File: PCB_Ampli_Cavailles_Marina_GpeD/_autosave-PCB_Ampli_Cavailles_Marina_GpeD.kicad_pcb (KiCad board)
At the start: 2 copper layers, 52 parts, among them J2 Conn_01x02, J3 Conn_01x03, Q1 2N2907, Q10 TIP32, Q11 BD138, Q12 TIP31, Q13 2N2222, Q2 2N2907, Q3 2N2907, Q4 2N2222, Q5 2N2222, Q6 2N2907, Q7 2N2907, Q8 BD139, Q9 BD139, U1 Relay_1CT, U2 Jack_Mono

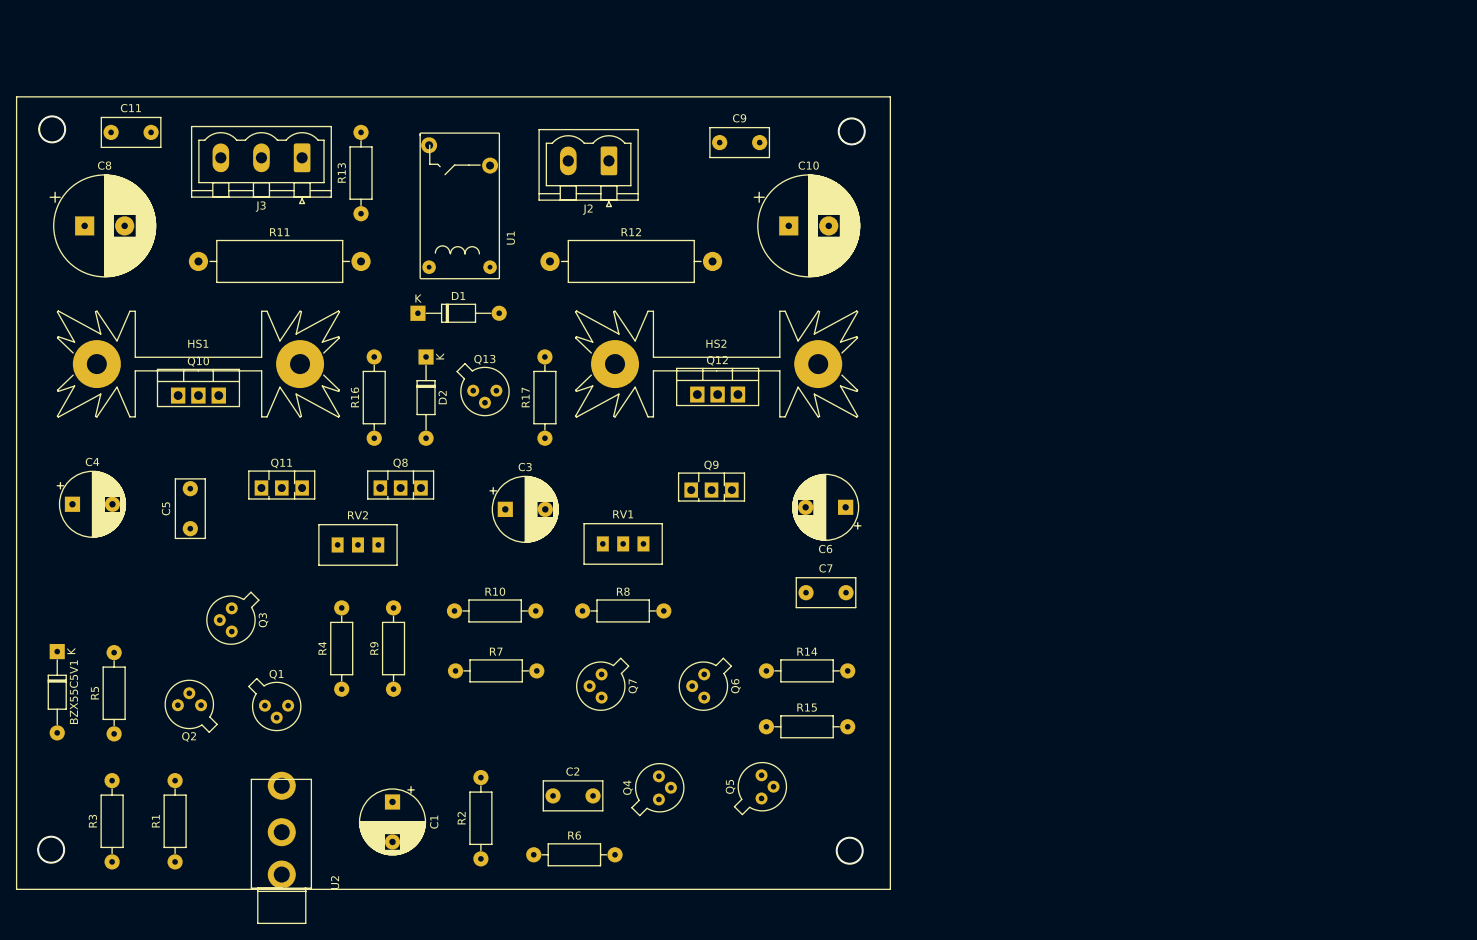
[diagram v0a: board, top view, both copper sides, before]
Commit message: PCB modifié
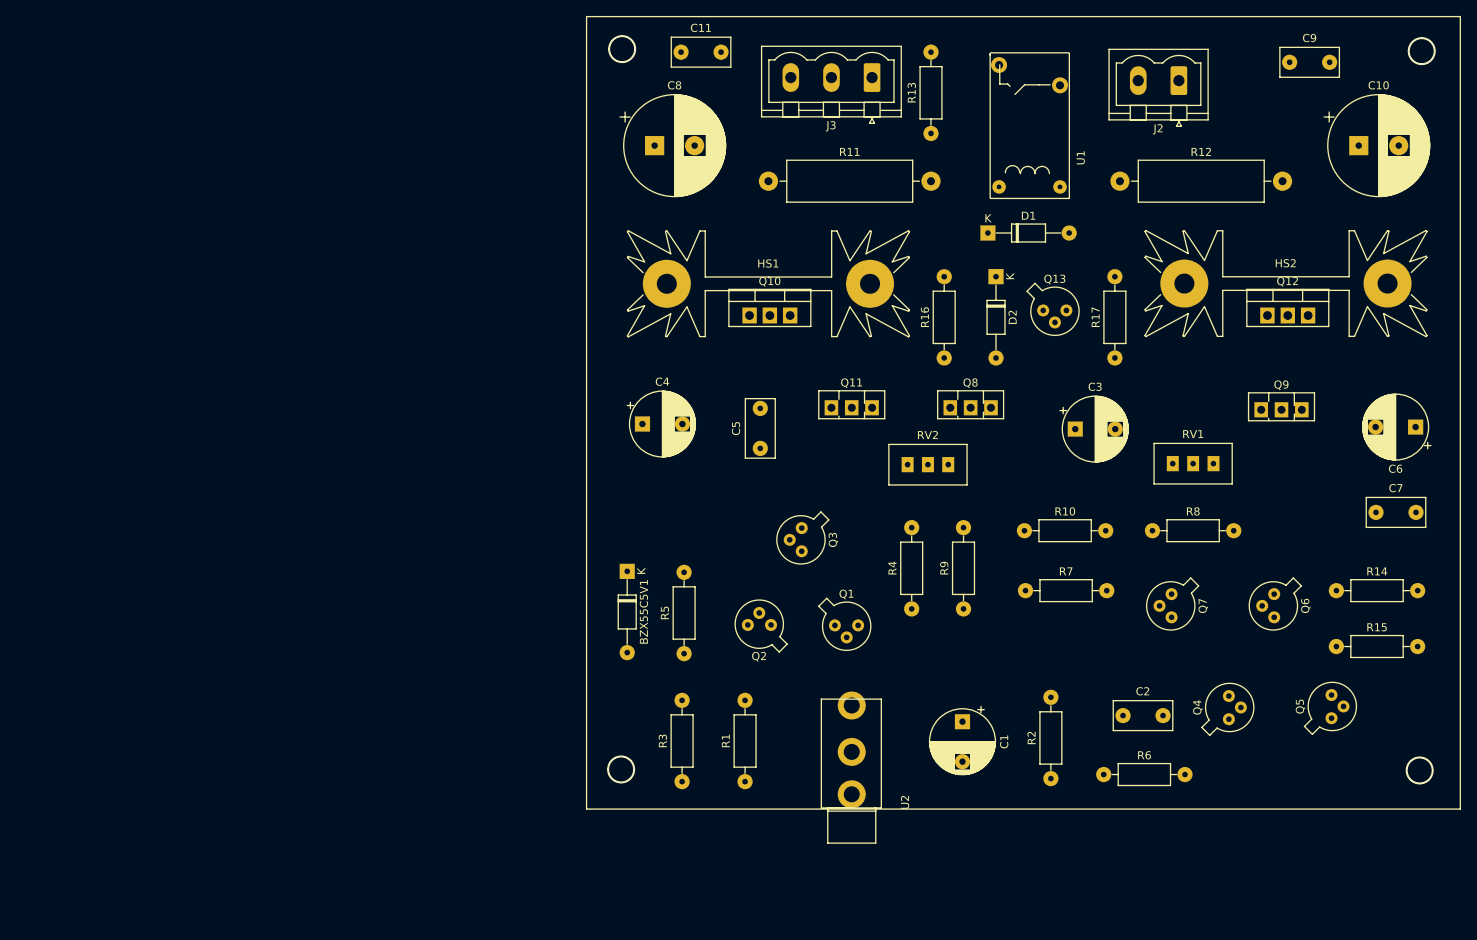
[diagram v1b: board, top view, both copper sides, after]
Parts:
- moved Q10 72.1 mm to (117.0, 80.7)
- moved Q12 72.0 mm to (181.8, 80.7)
- moved C3 71.9 mm to (157.7, 94.9)
- moved C4 71.9 mm to (103.6, 94.2)
- moved C5 71.9 mm to (118.4, 97.3)
- moved C8 71.9 mm to (105.2, 59.4)
- moved D1 71.9 mm to (146.8, 70.4)
- moved Q11 71.9 mm to (127.3, 92.2)
- moved Q2 71.9 mm to (119.5, 119.3)
- moved Q4 71.9 mm to (177.0, 130.9)
- moved Q5 71.9 mm to (189.9, 130.8)
- moved R17 71.9 mm to (162.7, 86.0)
- moved R2 71.9 mm to (154.7, 138.6)
- moved R9 71.9 mm to (143.8, 117.3)
- moved RV2 71.9 mm to (141.9, 99.3)
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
